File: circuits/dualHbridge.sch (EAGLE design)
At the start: 32 parts, among them Q1 FDS5680, Q2 FDS5680, Q3 FDS5680, Q4 FDS5680, Q5 FDS5680, Q6 FDS5680, Q7 FDS5680, Q8 FDS5680

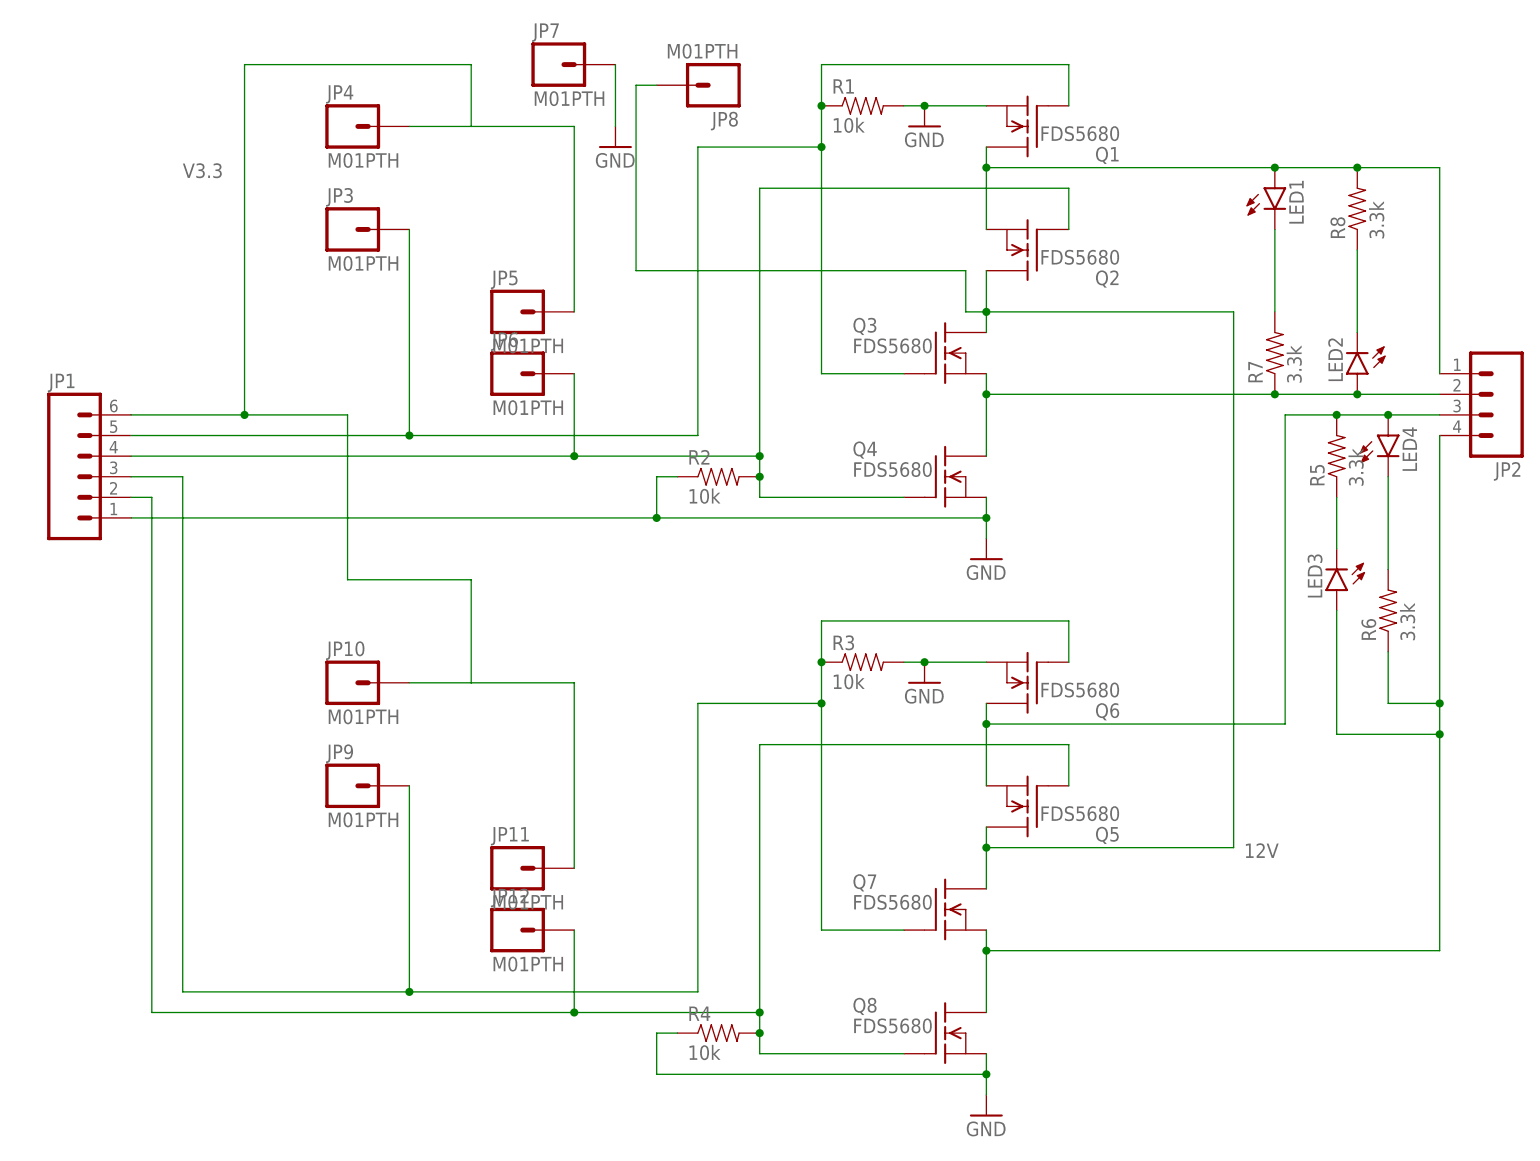
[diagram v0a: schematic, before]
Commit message: h bridge circuit board
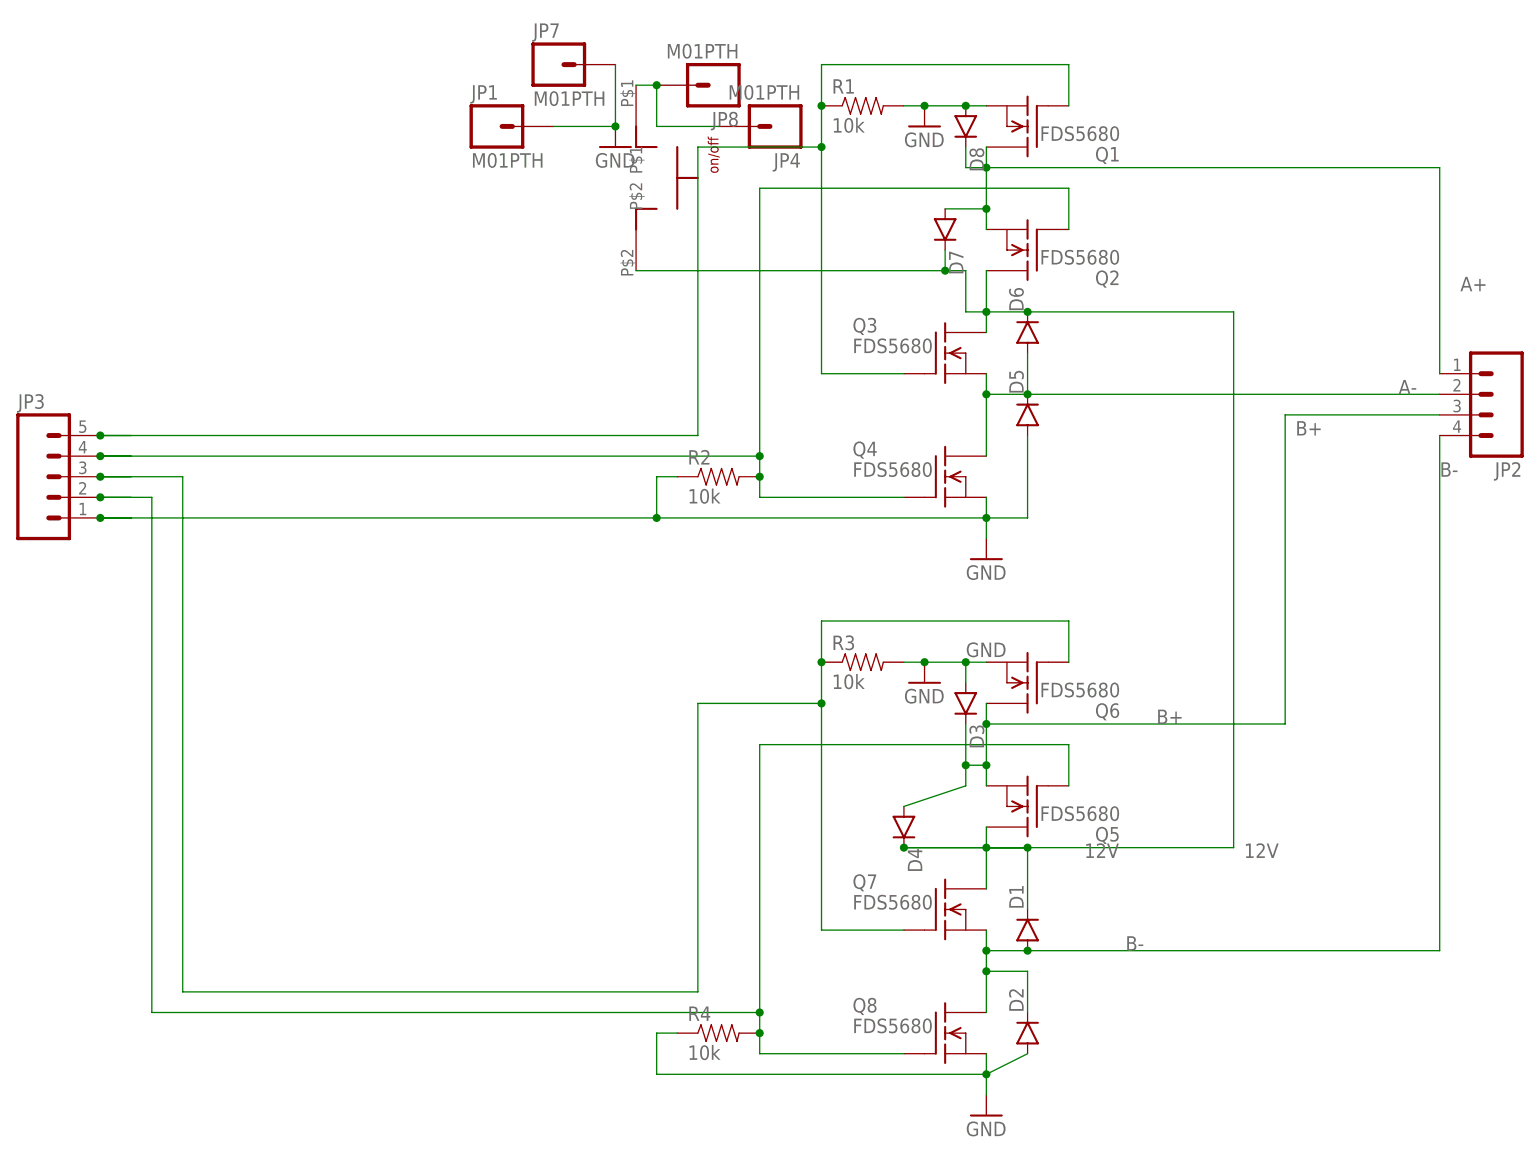
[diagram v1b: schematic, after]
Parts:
- removed JP10, JP11, JP12, JP5, JP6, JP9: M01PTH, SparkFun-Connectors:M01PTH
- removed LED1, LED2, LED3, LED4: (no value), SparkFun-LED:LED3MM
- removed R5, R6, R7, R8: 3.3k, SparkFun-Passives:RESISTOR0603-RES
- added D1, D2, D3, D4, D5, D6, D7, D8: (no value), SparkFun-DiscreteSemi:DIODEKIT2
- added U$5: CW182-ND, spietz-library:CW182-ND
- JP1: value (none) -> M01PTH; device SparkFun-Connectors:M06NO_SILK -> SparkFun-Connectors:M01PTH
- JP3: value M01PTH -> (none); device SparkFun-Connectors:M01PTH -> SparkFun-Connectors:M05PTH
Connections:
- removed net N$1: LED1.C, R7.2
- removed net N$10: LED4.C, R6.2
- removed net N$11: JP2.4, LED3.A, Q7.S, Q8.D, R6.1
- removed net N$12: JP2.3, LED4.A, Q5.S, Q6.D, R5.2
- removed net N$4: JP2.2, LED2.A, Q3.S, Q4.D, R7.1
- removed net N$5: JP2.1, LED1.A, Q1.D, Q2.S, R8.2
- removed net N$8: LED2.C, R8.1
- removed net N$9: LED3.C, R5.1
- removed net V3.3: JP1.6, JP10.1, JP11.1, JP4.1, JP5.1
- new net A+: D7.A, D8.C, JP2.1, Q1.D, Q2.S
- new net A-: D5.C, D6.A, JP2.2, Q3.S, Q4.D
- new net B+: D3.C, D4.A, JP2.3, Q5.S, Q6.D
- new net B-: D1.A, D2.C, JP2.4, Q7.S, Q8.D
- new net N$15: JP4.1, JP8.1, U$5.P$1
- net 12V: now also D1.C, D4.C, D6.C, D7.C, U$5.P$2; no longer JP8.1
- net GND: now also D2.A, D3.A, D5.A, D8.A, JP3.1
- net N$13: now also JP3.3; no longer JP1.3, JP9.1
- net N$14: now also JP3.2; no longer JP1.2, JP12.1
- net N$6: now also JP3.5; no longer JP1.5, JP3.1
- net N$7: now also JP3.4; no longer JP1.4, JP6.1
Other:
- moved on the sheet: JP4
